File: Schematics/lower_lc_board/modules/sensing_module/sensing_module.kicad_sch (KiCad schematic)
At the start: 21 parts, among them J4 HALL-1, J5 HALL-2, Q3 2N7002, U11 SI2301CDS-T1-GE3, U9 ADC_ADS131M04IPWR

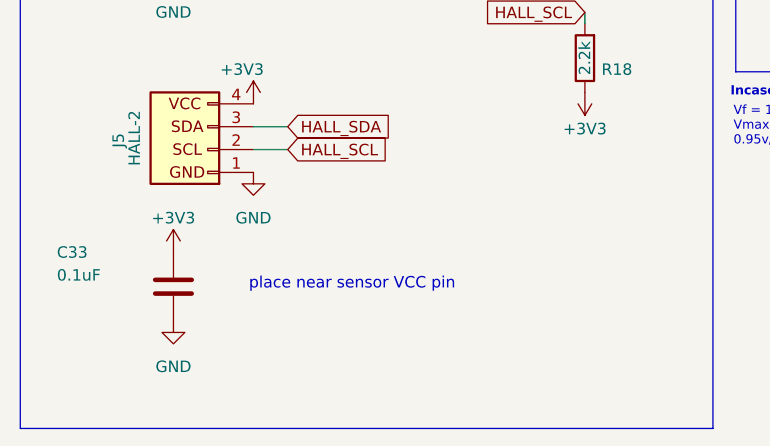
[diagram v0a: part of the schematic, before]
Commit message: organizational work
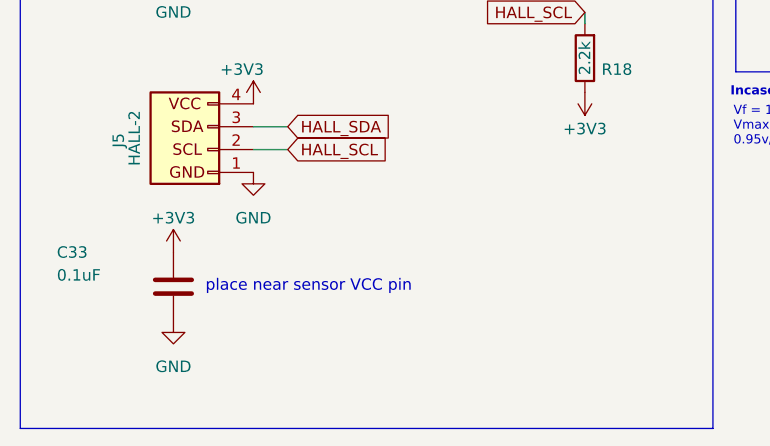
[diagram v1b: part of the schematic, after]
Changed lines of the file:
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@@
 	(text "place near sensor VCC pin"
 		(exclude_from_sim no)
-		(at 54.102 169.926 0)
+		(at 49.276 170.18 0)
 		(effects
 			(font
